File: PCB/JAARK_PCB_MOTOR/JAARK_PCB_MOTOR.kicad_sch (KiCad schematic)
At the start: 38 parts, among them IC1 TPS564242DRLR, IC10 DRV8231DDAR, IC9 DRV8231DDAR, J1 Battery Terminal, J2 Morpho_x2_SSW-119-01-T-D, J3 HC-05, J4 Metal Detector, Q1 SSM3J334RLF, Q3 BC237B, U1 4A

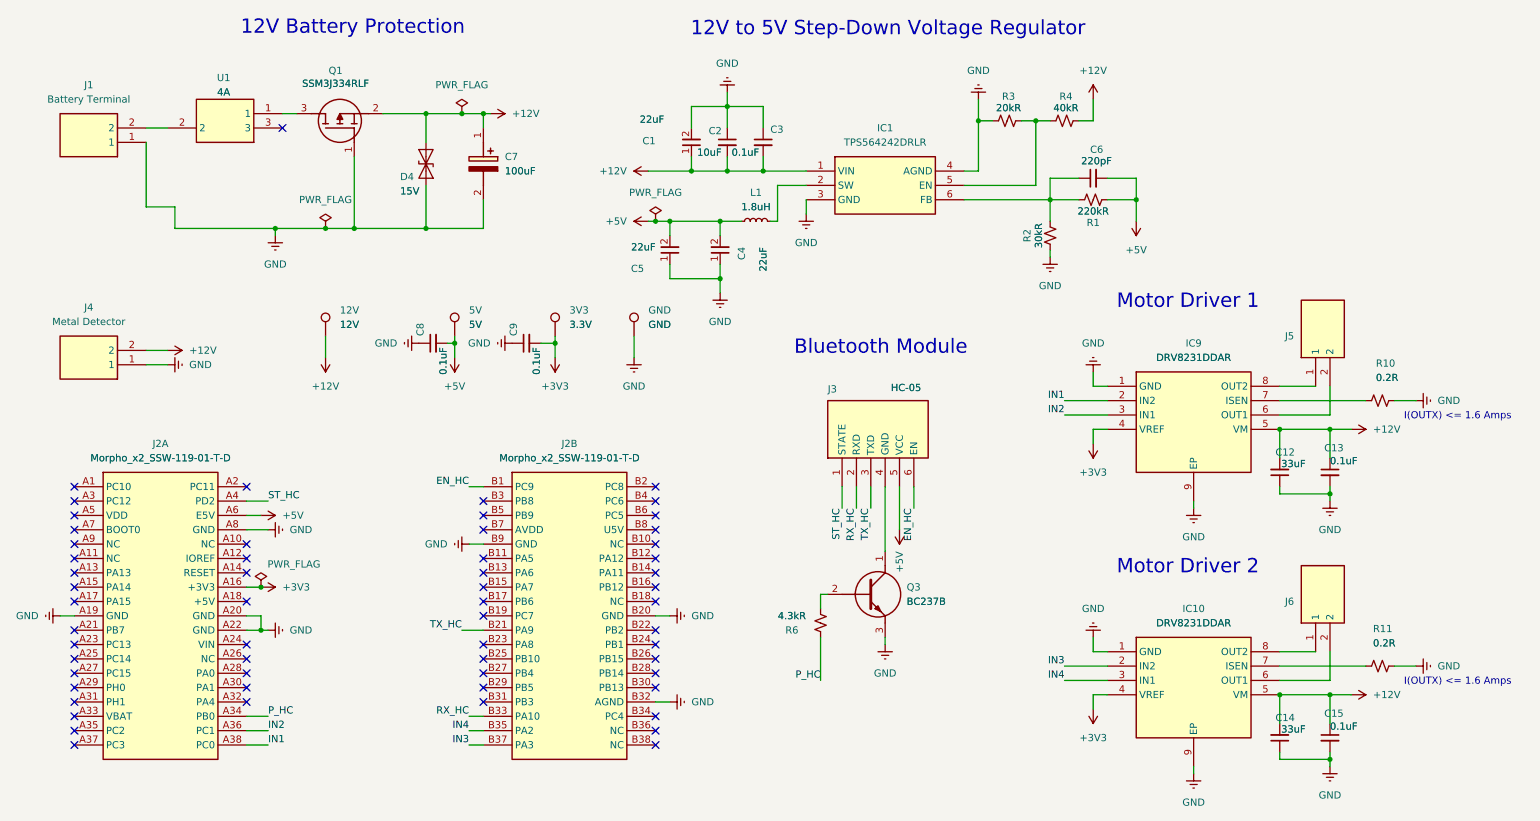
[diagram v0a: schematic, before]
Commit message: Final prototype of PCB
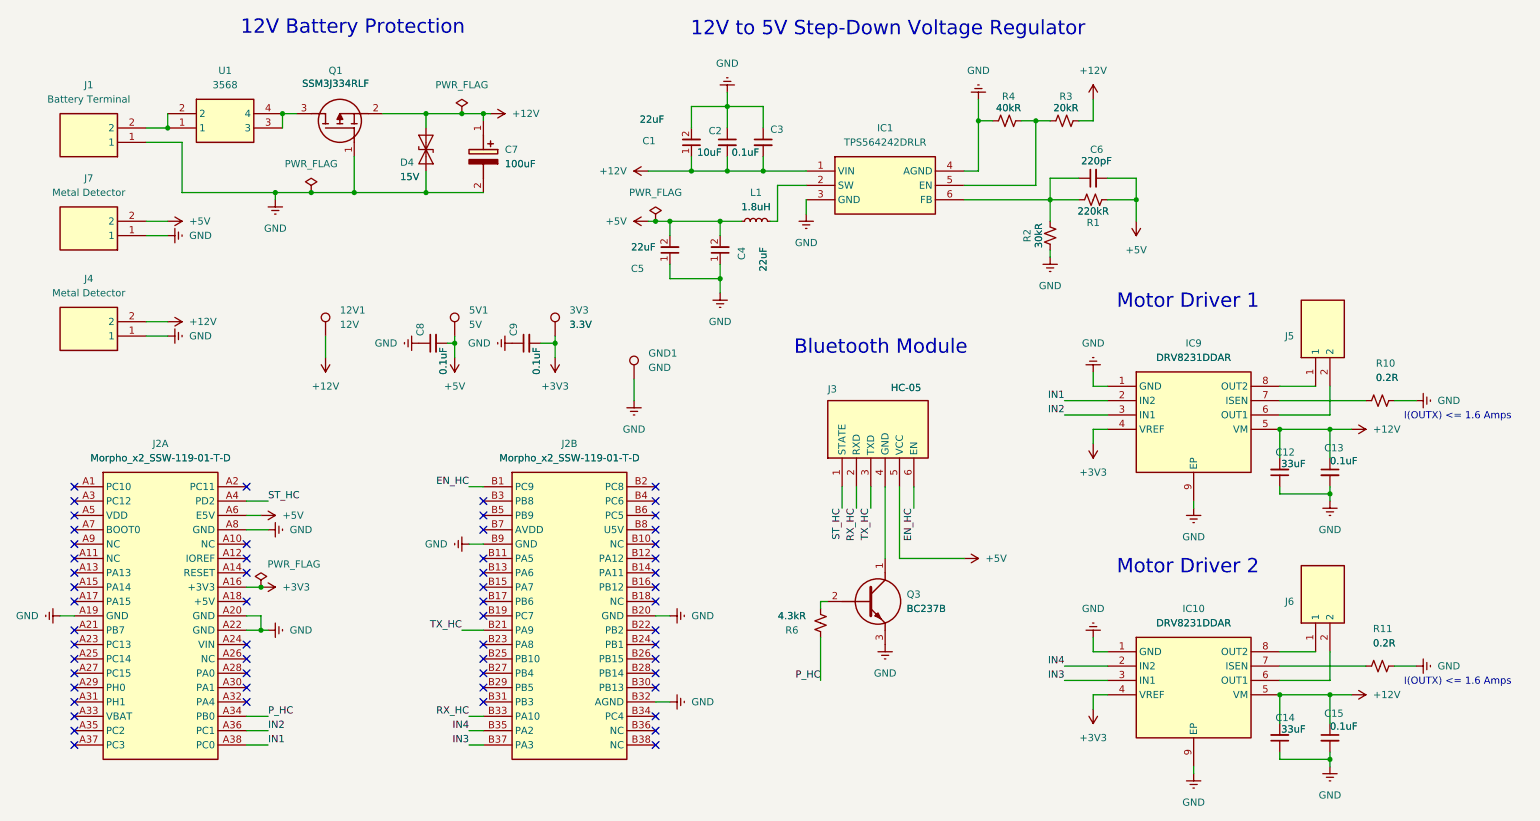
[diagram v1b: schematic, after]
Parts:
- removed U1: 4A, JAARK_lib:3586TR, symbol JAARK_lib:3586TR
- added J7: Metal Detector, JAARK_lib:1984617, symbol SSys_Parts:1984617
- added U1: 3568, 3568, symbol JAARK_lib:3568
- renumbered 12V to 12V1, 5V to 5V1, GND to GND1
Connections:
- net +12V: now also R3.1; no longer R4.1
- net +5V: now also J7.2
- net GND: now also R4.2, J7.1; no longer R3.2
- net IN3: now also IC10.3 (IN1); no longer IC10.2 (IN2)
- net IN4: now also IC10.2 (IN2); no longer IC10.3 (IN1)
- net at J1.2: now also U1.1, U1.2
- net at Q1.3 (D): now also U1.3, U1.4
- new net: IC1.5 (EN), R3.2, R4.1
- no-connect marks 59 -> 58
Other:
- moved on the sheet: C7, D4, GND1, J4, Q3, R3, R4
